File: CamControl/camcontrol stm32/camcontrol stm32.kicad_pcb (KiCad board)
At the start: 4 copper layers, 15.9 x 33.8 mm, 54 parts, among them J1 Power 1, J2 Conn_01x04, J3 Power 1, J4 Power 1, J5 Conn_01x06, J6 Conn_01x02, J7 Power 1, Q1 AO3401A, U1 BGS12P2L6, U2 BALFHB-WL-02D3, U3 STM32WLE4CCUx, U4 DS8242, U5 TPS25970LRPWR, U6 TPS25970LRPWR, U7 INA2180, Y1 32MHz

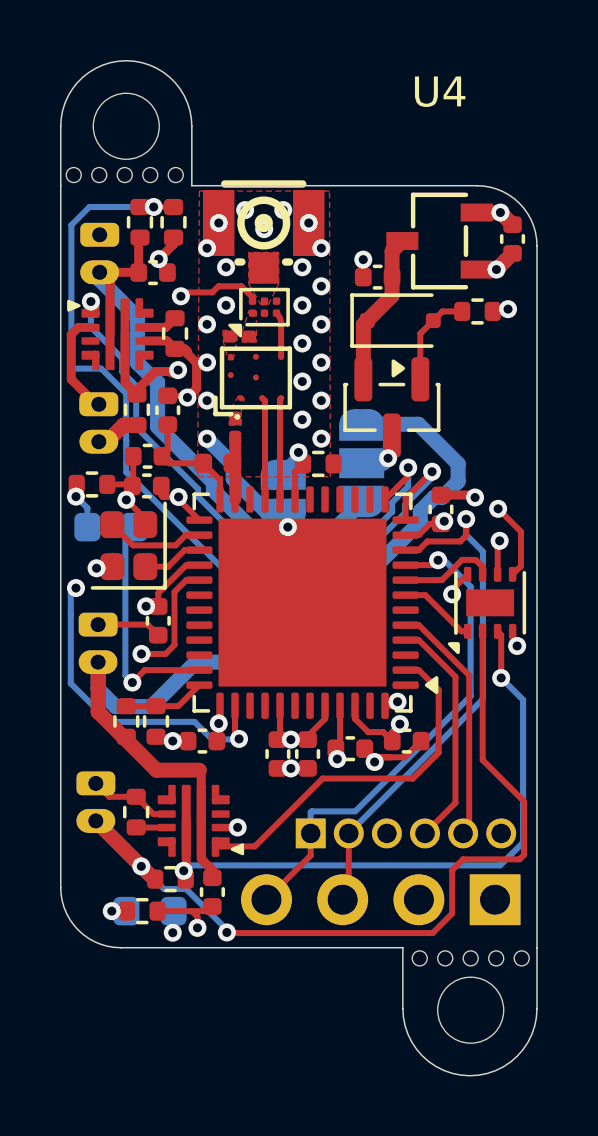
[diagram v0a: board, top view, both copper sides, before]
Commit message: fixed dumb issue
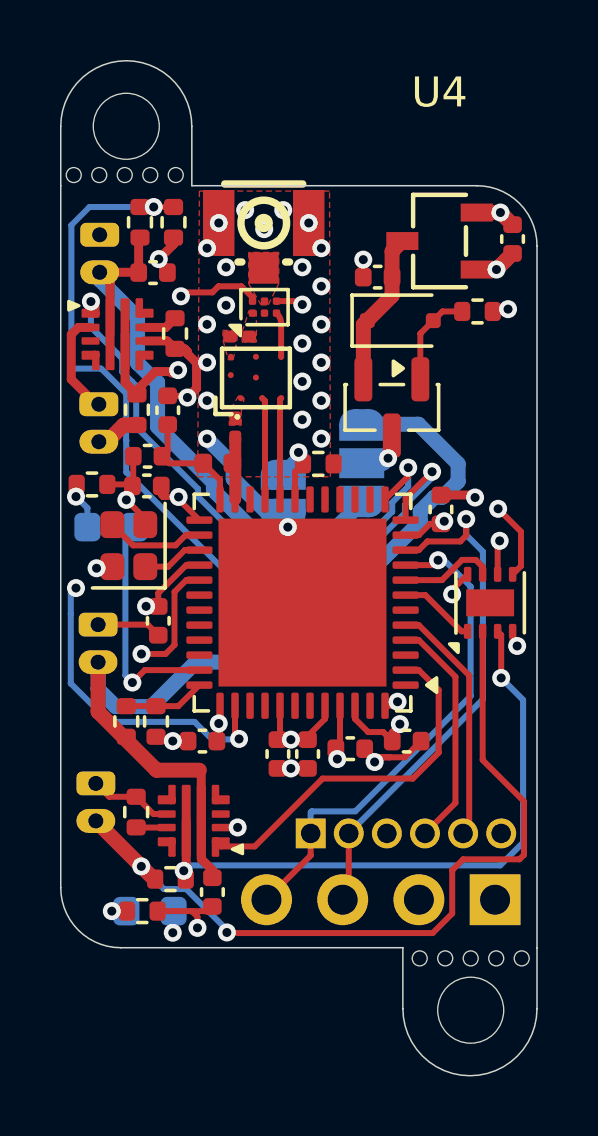
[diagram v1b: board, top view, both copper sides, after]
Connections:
- U1 pad 4: unconnected-(U1-VDD-Pad4) -> +3V3
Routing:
- net +3V3: track 16.4 -> 17.3 mm, vias 9 -> 10
- net GND: vias 39 -> 38
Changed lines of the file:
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@@
 	(net 65 "unconnected-(U3-PA6-Pad14)")
 	(net 66 "unconnected-(U3-PB0-Pad30)")
-	(net 67 "unconnected-(U1-VDD-Pad4)")
-	(net 68 "/RF CTRL")
+	(net 67 "/RF CTRL")
 	(footprint "Panelization:BreakLine_5h_D0.5mm_P0.85mm"
 		(layer "F.Cu")
@@
 			(layers "F.Cu" "F.Mask" "F.Paste")
 			(roundrect_rratio 0.25)
-			(net 68 "/RF CTRL")
+			(net 67 "/RF CTRL")
 			(pinfunction "PC13")
 			(pintype "bidirectional")
@@
 			(layers "F.Cu" "F.Mask")
 			(roundrect_rratio 0.25)
-			(net 67 "unconnected-(U1-VDD-Pad4)")
+			(net 2 "+3V3")
 			(pinfunction "VDD")
 			(pintype "power_in")
@@
 			(layers "F.Cu" "F.Mask")
 			(roundrect_rratio 0.25)
-			(net 68 "/RF CTRL")
+			(net 67 "/RF CTRL")
 			(pinfunction "CTRL")
 			(pintype "input")
@@
 	)
 	(via
-		(at 167.005 123.825)
-		(size 0.6)
-		(drill 0.3)
-		(layers "F.Cu" "B.Cu")
-		(free yes)
-		(net 1)
-	)
-	(via
 		(at 166.5224 131.2164)
 		(size 0.6)
@@
 	)
 	(segment
+		(start 166.8905 123.6851)
+		(end 167.005 123.7996)
+		(width 0.2)
+		(layer "F.Cu")
+		(net 2)
+	)
+	(segment
 		(start 169.203101 138.049)
 		(end 169.7034 138.049)
@@
 	)
 	(segment
+		(start 166.146 123.6851)
+		(end 166.8905 123.6851)
+		(width 0.2)
+		(layer "F.Cu")
+		(net 2)
+	)
+	(segment
 		(start 163.5746 130.983)
 		(end 162.881551 130.289951)
@@
 		(net 2)
 	)
+	(via
+		(at 167.005 123.7996)
+		(size 0.6)
+		(drill 0.3)
+		(layers "F.Cu" "B.Cu")
+		(net 2)
+	)
 	(segment
 		(start 162.7125 144.7117)
@@
 		(width 0.2)
 		(layer "F.Cu")
-		(net 68)
+		(net 67)
 	)
 	(segment
@@
 		(width 0.2)
 		(layer "F.Cu")
-		(net 68)
+		(net 67)
 	)
 	(segment
@@
 		(width 0.2)
 		(layer "F.Cu")
-		(net 68)
+		(net 67)
 	)
 	(segment
@@
 		(width 0.2)
 		(layer "F.Cu")
-		(net 68)
+		(net 67)
 	)
 	(segment
@@
 		(width 0.2)
 		(layer "F.Cu")
-		(net 68)
+		(net 67)
 	)
 	(segment
@@
 		(width 0.2)
 		(layer "F.Cu")
-		(net 68)
+		(net 67)
 	)
 	(segment
@@
 		(width 0.2)
 		(layer "F.Cu")
-		(net 68)
+		(net 67)
 	)
 	(segment
@@
 		(width 0.2)
 		(layer "F.Cu")
-		(net 68)
+		(net 67)
 	)
 	(via
@@
 		(drill 0.3)
 		(layers "F.Cu" "B.Cu")
-		(net 68)
+		(net 67)
 	)
 	(via
@@
 		(drill 0.3)
 		(layers "F.Cu" "B.Cu")
-		(net 68)
+		(net 67)
 	)
 	(via
@@
 		(drill 0.3)
 		(layers "F.Cu" "B.Cu")
-		(net 68)
+		(net 67)
 	)
 	(segment
@@
 		(width 0.2)
 		(layer "B.Cu")
-		(net 68)
+		(net 67)
 	)
 	(segment
@@
 		(width 0.2)
 		(layer "B.Cu")
-		(net 68)
+		(net 67)
 	)
 	(segment
@@
 		(width 0.2)
 		(layer "B.Cu")
-		(net 68)
+		(net 67)
 	)
 	(segment
@@
 		(width 0.2)
 		(layer "B.Cu")
-		(net 68)
+		(net 67)
 	)
 	(segment
@@
 		(width 0.2)
 		(layer "B.Cu")
-		(net 68)
+		(net 67)
 	)
 	(segment
@@
 		(width 0.2)
 		(layer "B.Cu")
-		(net 68)
+		(net 67)
 	)
 	(segment
@@
 		(width 0.2)
 		(layer "B.Cu")
-		(net 68)
+		(net 67)
 	)
 	(segment
@@
 		(width 0.2)
 		(layer "B.Cu")
-		(net 68)
+		(net 67)
 	)
 	(segment
@@
 		(width 0.2)
 		(layer "In2.Cu")
-		(net 68)
+		(net 67)
 	)
 	(segment
@@
 		(width 0.2)
 		(layer "In2.Cu")
-		(net 68)
+		(net 67)
 	)
 	(segment
@@
 		(width 0.2)
 		(layer "In2.Cu")
-		(net 68)
+		(net 67)
 	)
 	(segment
@@
 		(width 0.2)
 		(layer "In2.Cu")
-		(net 68)
+		(net 67)
 	)
 	(segment
@@
 		(width 0.2)
 		(layer "In2.Cu")
-		(net 68)
+		(net 67)
 	)
 	(segment
@@
 		(width 0.2)
 		(layer "In2.Cu")
-		(net 68)
+		(net 67)
 	)
 	(segment
@@
 		(width 0.2)
 		(layer "In2.Cu")
-		(net 68)
+		(net 67)
 	)
 	(zone

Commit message: nvm i missed it up
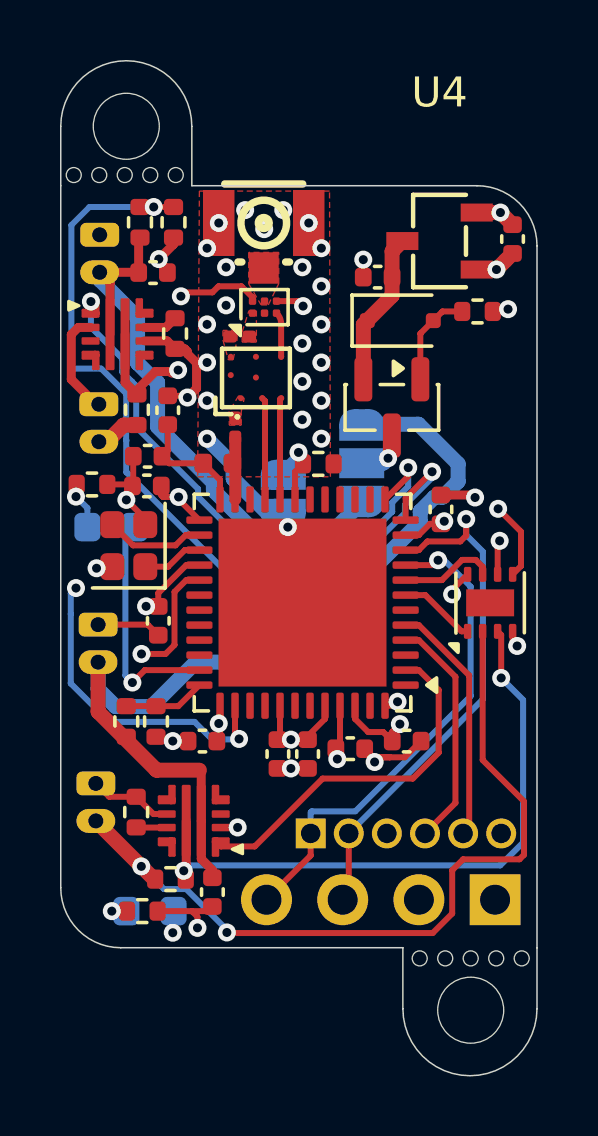
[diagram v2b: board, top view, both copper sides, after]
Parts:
- R3, R5: value 20m -> 10m
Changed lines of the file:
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@@
 			)
 		)
-		(property "Value" "20m"
+		(property "Value" "10m"
 			(at 0 1.17 90)
 			(layer "F.Fab")
@@
 			)
 		)
+		(property "LCSC Part" "C3024467"
+			(at 0 0 270)
+			(unlocked yes)
+			(layer "F.Fab")
+			(hide yes)
+			(effects
+				(font
+					(size 1 1)
+					(thickness 0.15)
+				)
+			)
+		)
 		(property ki_fp_filters "R_*")
 		(sheetname "/")
@@
 			)
 		)
+		(property "LCSC Part" "C14441"
+			(at 0 0 180)
+			(unlocked yes)
+			(layer "F.Fab")
+			(hide yes)
+			(effects
+				(font
+					(size 1 1)
+					(thickness 0.15)
+				)
+			)
+		)
 		(property ki_fp_filters "C_*")
 		(sheetname "/")
@@
 			)
 		)
+		(property "LCSC Part" "C5142571"
+			(at 0 0 270)
+			(unlocked yes)
+			(layer "F.Fab")
+			(hide yes)
+			(effects
+				(font
+					(size 1 1)
+					(thickness 0.15)
+				)
+			)
+		)
 		(property ki_fp_filters "C_*")
 		(sheetname "/")
@@
 			)
 		)
+		(property "LCSC Part" "C5142571"
+			(at 0 0 0)
+			(unlocked yes)
+			(layer "F.Fab")
+			(hide yes)
+			(effects
+				(font
+					(size 1 1)
+					(thickness 0.15)
+				)
+			)
+		)
 		(property ki_fp_filters "C_*")
 		(sheetname "/")
@@
 			)
 		)
+		(property "LCSC Part" "C3312945"
+			(at 0 0 90)
+			(unlocked yes)
+			(layer "F.Fab")
+			(hide yes)
+			(effects
+				(font
+					(size 1 1)
+					(thickness 0.15)
+				)
+			)
+		)
 		(property ki_fp_filters "*PG?TSNP*0.7x1.1mm*P0.4mm*")
 		(sheetname "/")
@@
 			)
 		)
-		(property "Value" "20m"
+		(property "Value" "10m"
 			(at 0 1.17 0)
 			(layer "F.Fab")
@@
 			)
 		)
+		(property "LCSC Part" "C3024467"
+			(at 0 0 180)
+			(unlocked yes)
+			(layer "F.Fab")
+			(hide yes)
+			(effects
+				(font
+					(size 1 1)
+					(thickness 0.15)
+				)
+			)
+		)
 		(property ki_fp_filters "R_*")
 		(sheetname "/")
@@
 			)
 		)
+		(property "LCSC Part" "C1546"
+			(at 0 0 270)
+			(unlocked yes)
+			(layer "F.Fab")
+			(hide yes)
+			(effects
+				(font
+					(size 1 1)
+					(thickness 0.15)
+				)
+			)
+		)
 		(property ki_fp_filters "C_*")
 		(sheetname "/")
@@
 	)
 	(segment
-		(start 166.8905 123.6851)
-		(end 167.005 123.7996)
-		(width 0.2)
-		(layer "F.Cu")
-		(net 2)
-	)
-	(segment
 		(start 169.203101 138.049)
 		(end 169.7034 138.049)
@@
 	)
 	(segment
+		(start 166.8651 123.6851)
+		(end 167.0304 123.8504)
+		(width 0.2)
+		(layer "F.Cu")
+		(net 2)
+	)
+	(segment
 		(start 162.2044 133.8606)
 		(end 162.2044 133.415701)
@@
 	(segment
 		(start 166.146 123.6851)
-		(end 166.8905 123.6851)
+		(end 166.8651 123.6851)
 		(width 0.2)
 		(layer "F.Cu")
@@
 	)
 	(via
-		(at 170.257721 137.78363)
+		(at 167.0304 123.8504)
 		(size 0.6)
 		(drill 0.3)
@@
 	)
 	(via
-		(at 162.687 144.7372)
+		(at 170.257721 137.78363)
 		(size 0.6)
 		(drill 0.3)
@@
 	)
 	(via
-		(at 166.624 138.3008)
+		(at 162.687 144.7372)
 		(size 0.6)
 		(drill 0.3)
@@
 	)
 	(via
-		(at 162.881551 130.212311)
+		(at 166.624 138.3008)
 		(size 0.6)
 		(drill 0.3)
@@
 	)
 	(via
-		(at 167.005 123.7996)
+		(at 162.881551 130.212311)
 		(size 0.6)
 		(drill 0.3)
